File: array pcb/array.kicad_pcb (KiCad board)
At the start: 2 copper layers, 218.3 x 76.2 mm, 170 parts

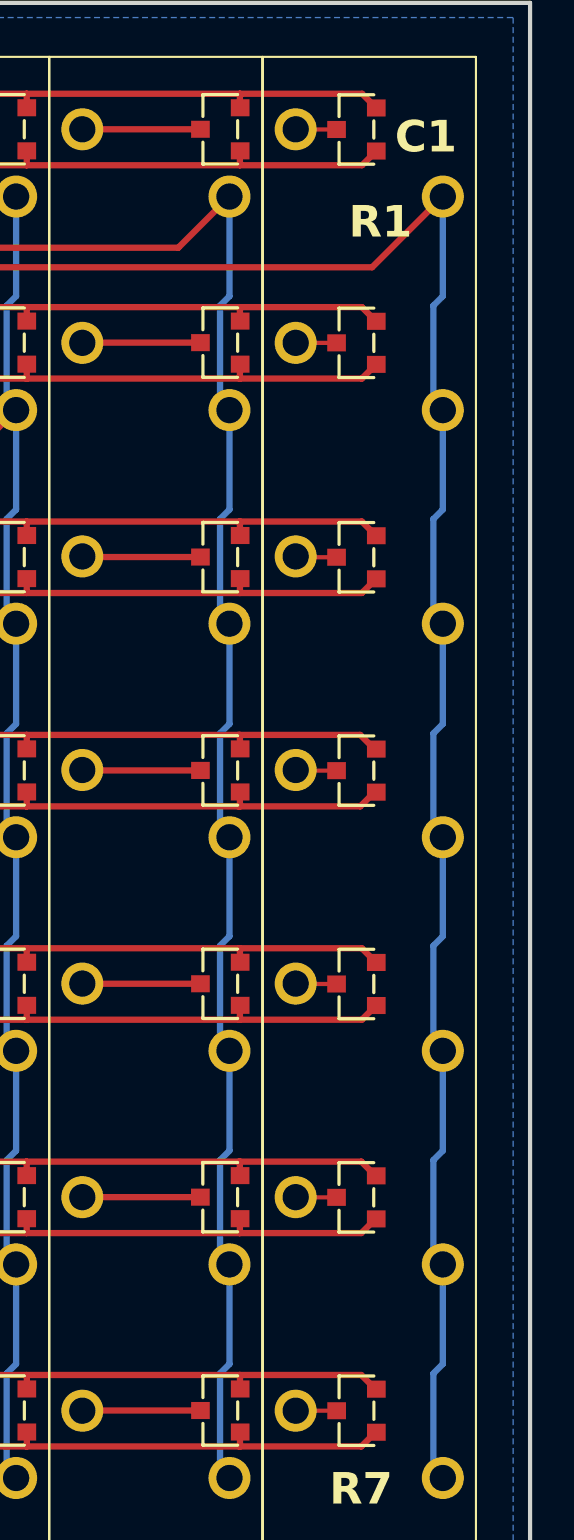
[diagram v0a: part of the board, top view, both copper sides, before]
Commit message: asd
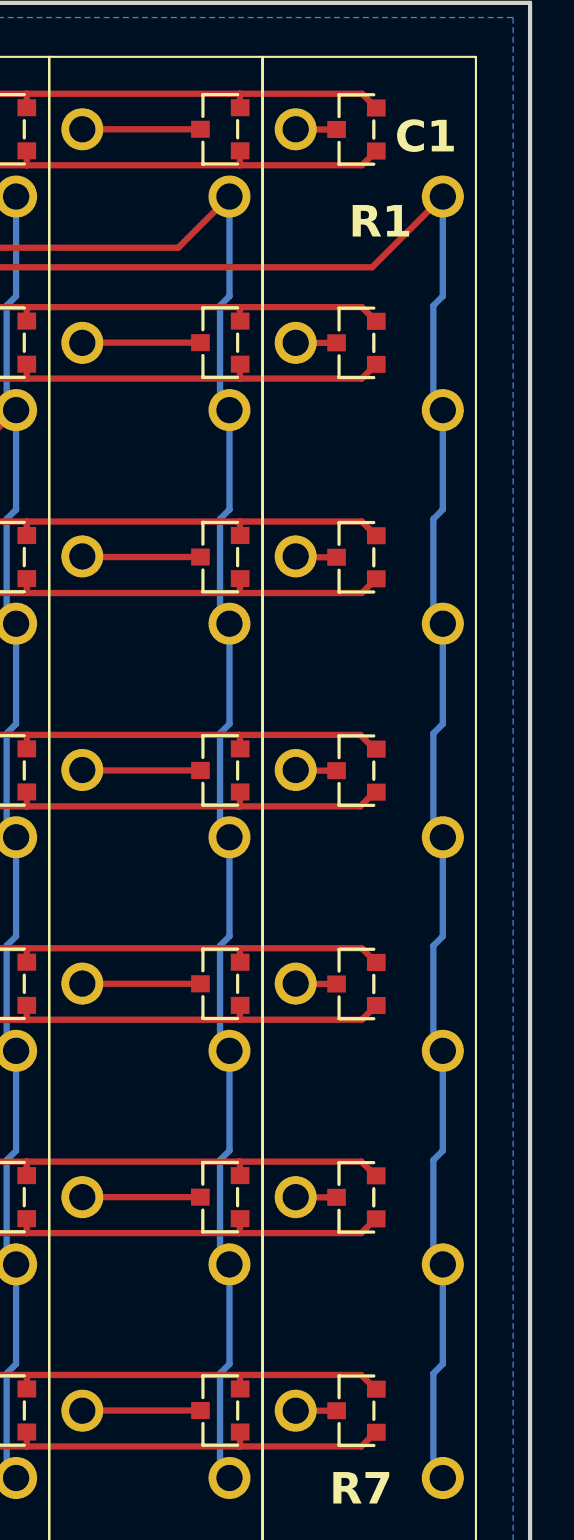
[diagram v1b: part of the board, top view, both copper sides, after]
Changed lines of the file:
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@@
 		(start 253.857502 91.485)
 		(end 251.922502 91.485)
-		(width 0.2)
+		(width 0.3)
 		(layer "F.Cu")
 		(net 0)
@@
 		(start 253.782502 81.335)
 		(end 251.847502 81.335)
-		(width 0.2)
+		(width 0.3)
 		(layer "F.Cu")
 		(net 0)
@@
 		(start 253.832502 101.635)
 		(end 251.897502 101.635)
-		(width 0.2)
+		(width 0.3)
 		(layer "F.Cu")
 		(net 0)
@@
 		(start 253.87 50.835)
 		(end 251.935 50.835)
-		(width 0.2)
+		(width 0.3)
 		(layer "F.Cu")
 		(net 0)
@@
 		(start 253.857502 71.185)
 		(end 251.922502 71.185)
-		(width 0.2)
+		(width 0.3)
 		(layer "F.Cu")
 		(net 0)
@@
 		(start 251.935 50.835)
 		(end 251.925 50.825)
-		(width 0.2)
+		(width 0.3)
 		(layer "F.Cu")
 		(net 0)
@@
 		(start 253.8575 60.985)
 		(end 251.9225 60.985)
-		(width 0.2)
+		(width 0.3)
 		(layer "F.Cu")
 		(net 0)
@@
 		(start 253.832502 111.785)
 		(end 251.897502 111.785)
-		(width 0.2)
+		(width 0.3)
 		(layer "F.Cu")
 		(net 0)

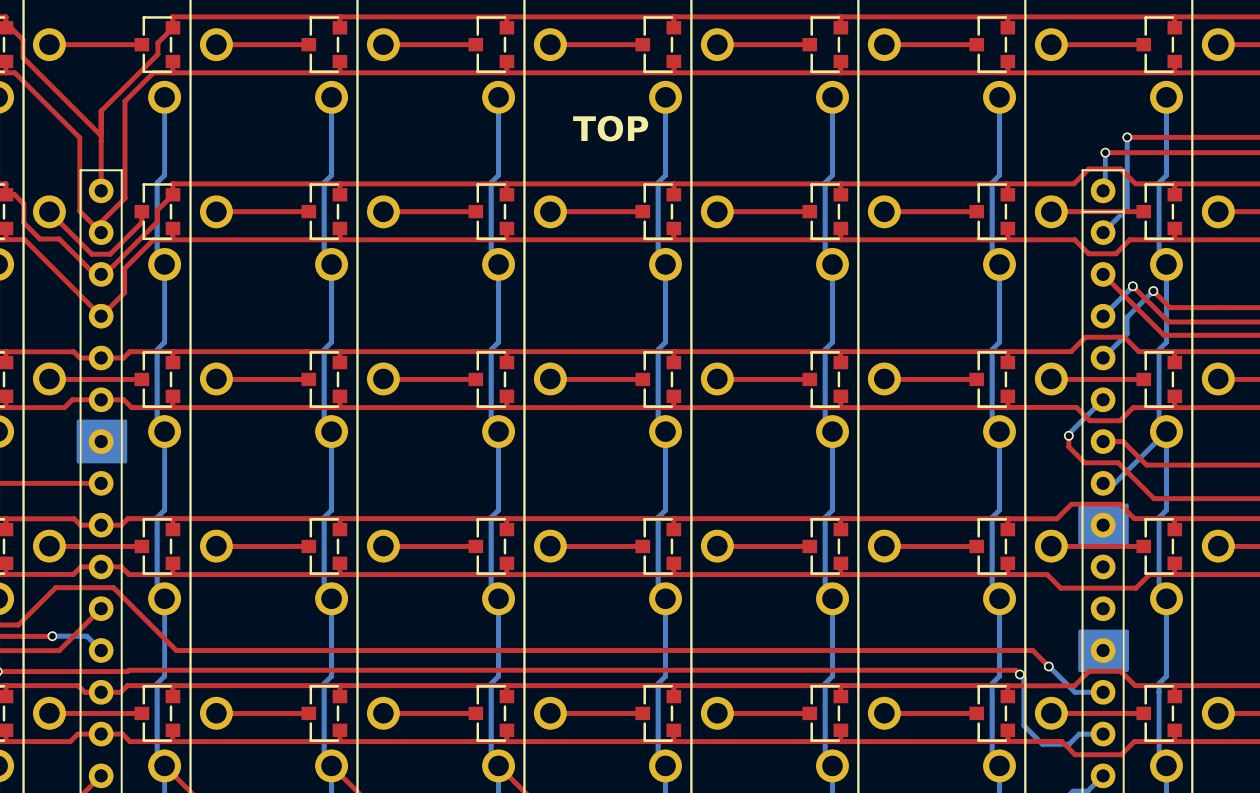
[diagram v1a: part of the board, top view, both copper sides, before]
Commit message: asd
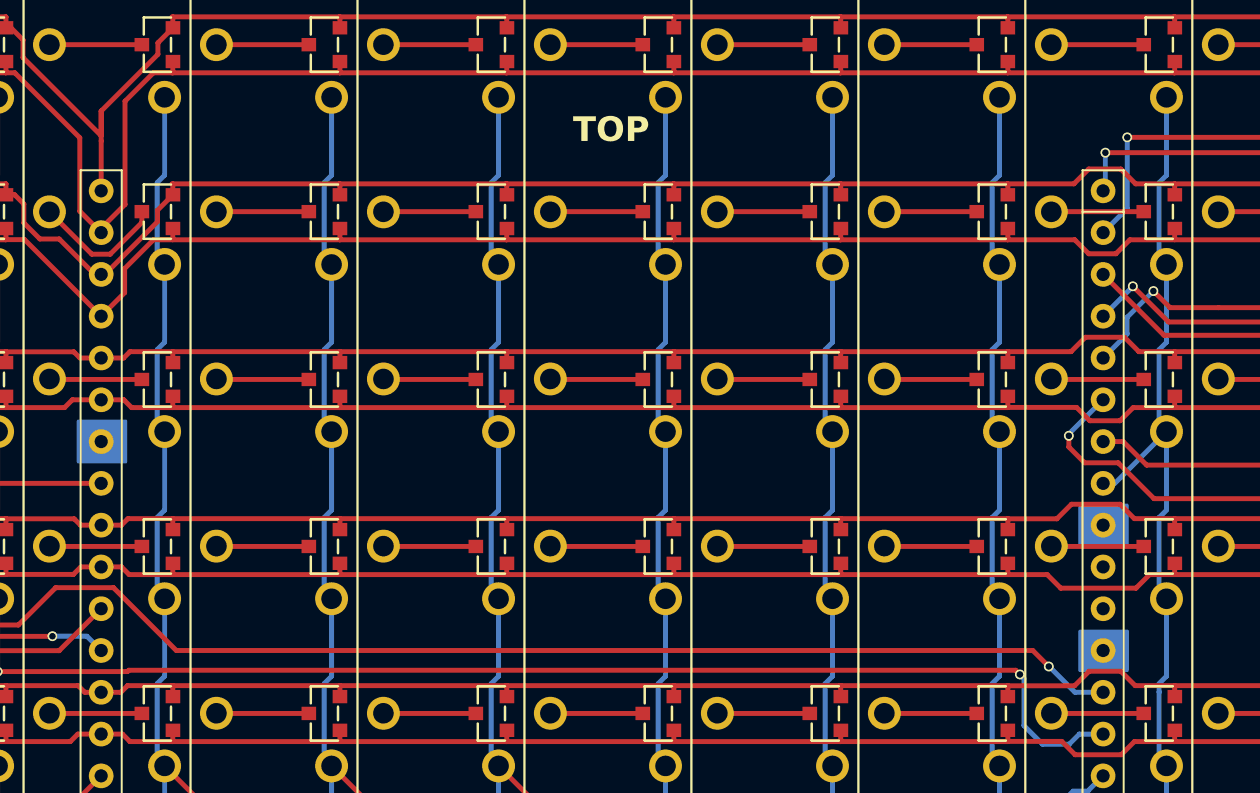
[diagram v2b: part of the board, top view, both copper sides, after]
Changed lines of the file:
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@@
 	)
 	(segment
-		(start 127.484999 51.849999)
-		(end 127.475 51.859998)
-		(width 0.3)
-		(layer "F.Cu")
-		(net 0)
-	)
-	(segment
 		(start 109.84 81.325)
 		(end 115.445 81.325)
@@
 	)
 	(segment
+		(start 124.5725 60.5375)
+		(end 123.1225 61.9875)
+		(width 0.3)
+		(layer "F.Cu")
+		(net 0)
+	)
+	(segment
 		(start 56.442499 49.140001)
 		(end 56.4475 49.135)
@@
 	)
 	(segment
+		(start 124.5725 54.26)
+		(end 124.5725 60.5375)
+		(width 0.3)
+		(layer "F.Cu")
+		(net 0)
+	)
+	(segment
 		(start 97.025 93.185)
 		(end 107.175 93.185)
@@
 	)
 	(segment
-		(start 124.5725 60.16)
-		(end 123.1225 61.61)
-		(width 0.3)
-		(layer "F.Cu")
-		(net 0)
-	)
-	(segment
 		(start 66.5475 83.035)
 		(end 66.5475 82.365)
@@
 	)
 	(segment
+		(start 123.1225 61.9875)
+		(end 123.1225 62.25)
+		(width 0.3)
+		(layer "F.Cu")
+		(net 0)
+	)
+	(segment
 		(start 97.034999 69.494999)
 		(end 97.025 69.485)
@@
 	)
 	(segment
-		(start 127.475 51.859998)
-		(end 127.475 52.535)
-		(width 0.3)
-		(layer "F.Cu")
-		(net 0)
-	)
-	(segment
 		(start 218.8225 59.285)
 		(end 228.9725 59.285)
@@
 	)
 	(segment
+		(start 127.475 51.859998)
+		(end 127.475 52.535)
+		(width 0.3)
+		(layer "F.Cu")
+		(net 0)
+	)
+	(segment
 		(start 150.4375 81.325)
 		(end 156.0425 81.325)
@@
 	)
 	(segment
+		(start 127.475 52.535)
+		(end 126.2975 52.535)
+		(width 0.3)
+		(layer "F.Cu")
+		(net 0)
+	)
+	(segment
 		(start 76.734999 59.294999)
 		(end 76.725 59.285)
@@
 	)
 	(segment
+		(start 126.2975 52.535)
+		(end 124.5725 54.26)
+		(width 0.3)
+		(layer "F.Cu")
+		(net 0)
+	)
+	(segment
 		(start 86.8775 110.740002)
 		(end 86.887499 110.750001)
@@
 	)
 	(segment
-		(start 127.475 52.535)
-		(end 126.2975 52.535)
-		(width 0.3)
-		(layer "F.Cu")
-		(net 0)
-	)
-	(segment
 		(start 59.0475 50.835)
 		(end 64.6525 50.835)
@@
 	)
 	(segment
-		(start 126.2975 52.535)
-		(end 124.5725 54.26)
-		(width 0.3)
-		(layer "F.Cu")
-		(net 0)
-	)
-	(segment
 		(start 187.7225 68.49)
 		(end 234.32 68.49)
@@
 	)
 	(segment
-		(start 123.1225 61.61)
-		(end 123.1225 62.25)
-		(width 0.3)
-		(layer "F.Cu")
-		(net 0)
-	)
-	(segment
 		(start 208.6725 72.885)
 		(end 208.6725 72.209998)
@@
 	)
 	(segment
-		(start 124.5725 54.26)
-		(end 124.5725 60.16)
-		(width 0.3)
-		(layer "F.Cu")
-		(net 0)
-	)
-	(segment
 		(start 150.4375 50.825)
 		(end 156.0425 50.825)
@@
 	)
 	(segment
+		(start 127.484999 51.849999)
+		(end 127.475 51.859998)
+		(width 0.3)
+		(layer "F.Cu")
+		(net 0)
+	)
+	(segment
 		(start 208.675 113.485)
 		(end 208.675 112.809998)
@@
 		(width 0.3)
 		(layer "B.Cu")
-		(net 0)
-	)
-	(segment
-		(start 187.42 90.19)
-		(end 187.425 90.185)
-		(width 0.3)
-		(layer "B.Cu")
